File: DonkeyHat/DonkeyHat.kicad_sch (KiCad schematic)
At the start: 12 parts, among them J1 GPIO, J2 Encoder 2, J3 Encoder 1, U2 rp2040-zero

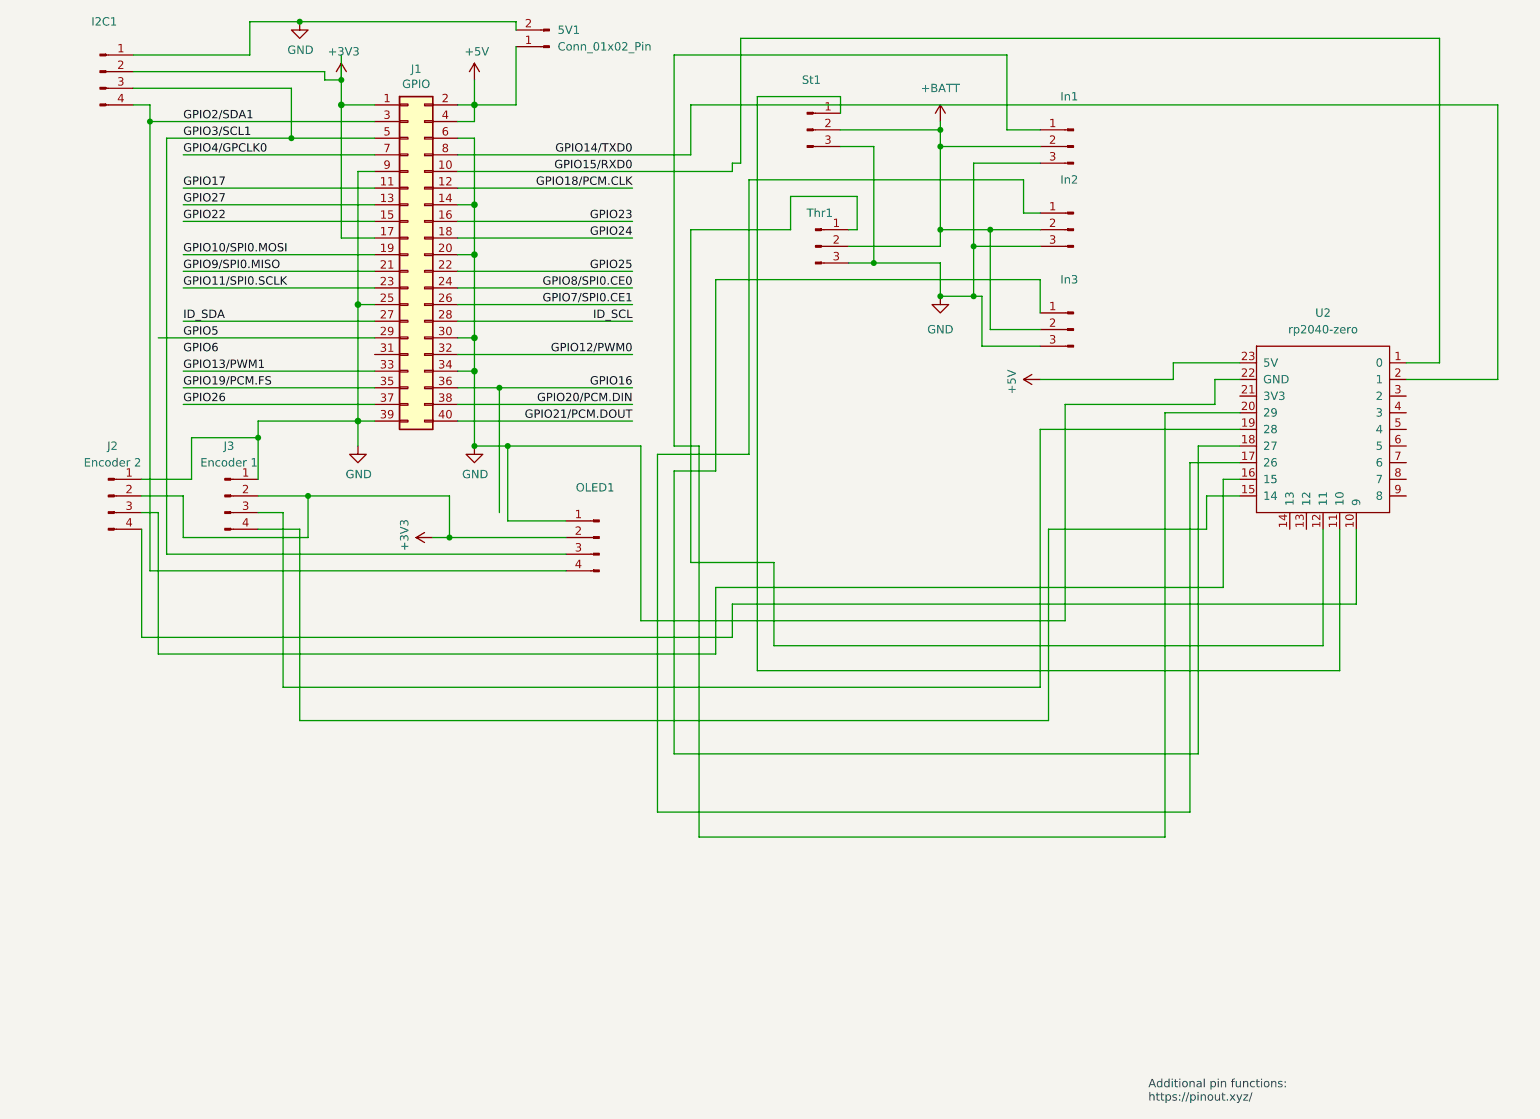
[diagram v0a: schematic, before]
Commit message: Typo
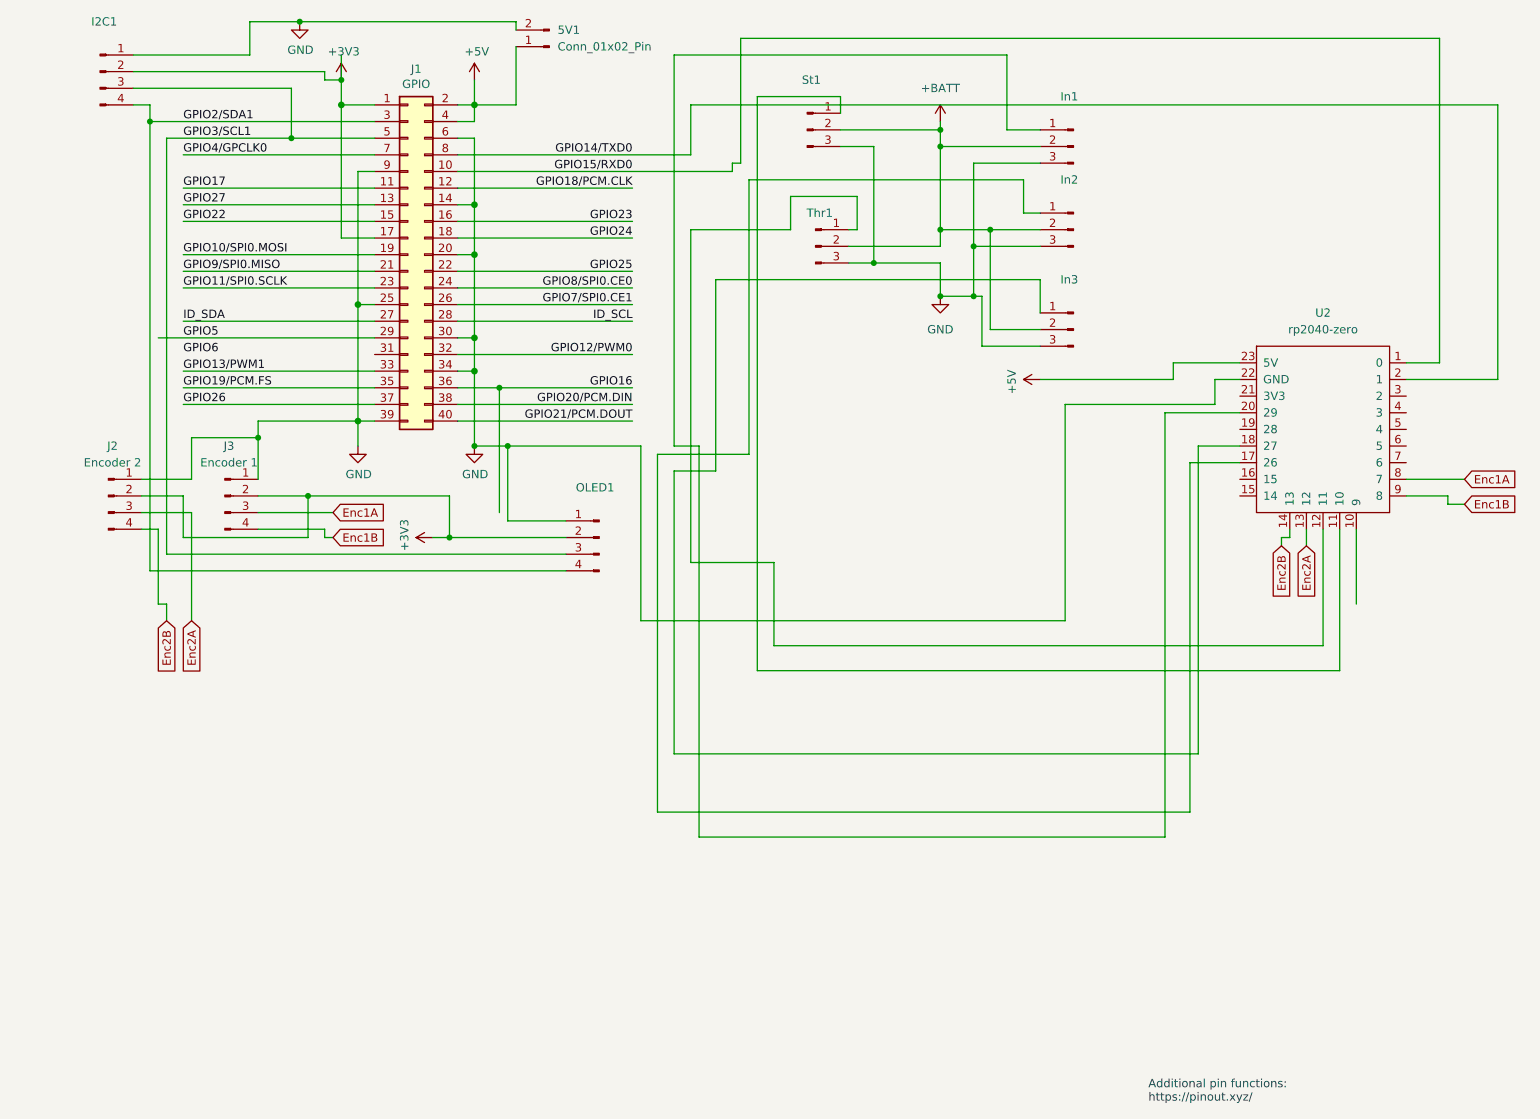
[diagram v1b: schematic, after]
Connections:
- net at U2.16 (15): no longer J2.3 (Pin_3)
- net at U2.10 (9): no longer J2.4 (Pin_4)
- net at U2.19 (28): no longer J3.3 (Pin_3)
- net at U2.15 (14): no longer J3.4 (Pin_4)
- net Enc2A: now reaches U2.13 (12)
- net Enc2A: now also J2.3 (Pin_3)
- net Enc2B: now reaches U2.14 (13)
- net Enc2B: now also J2.4 (Pin_4)
- net Enc1A: now reaches U2.8 (7)
- net Enc1A: now also J3.3 (Pin_3)
- net Enc1B: now reaches U2.9 (8)
- net Enc1B: now also J3.4 (Pin_4)

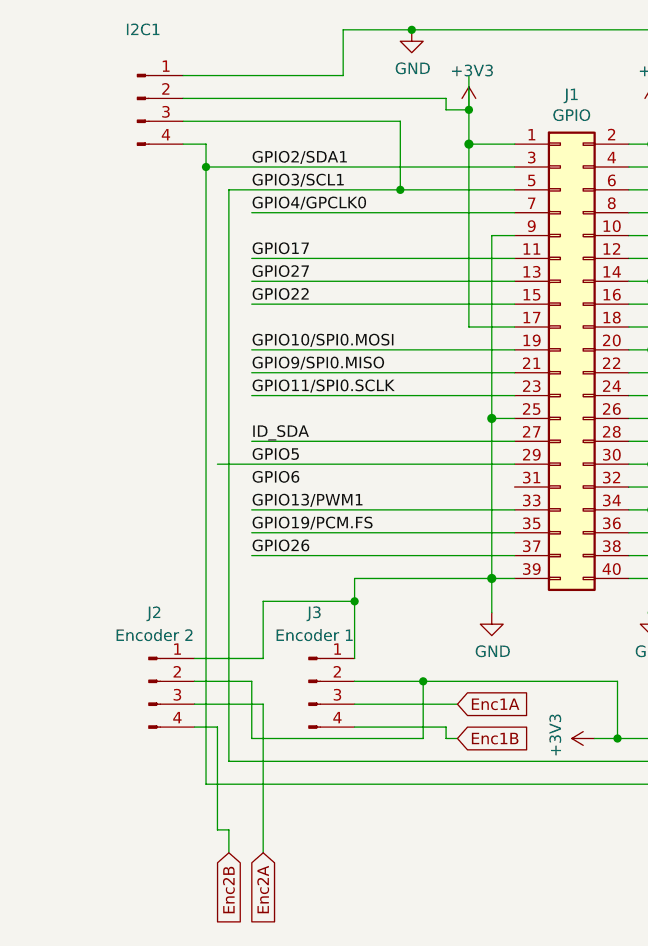
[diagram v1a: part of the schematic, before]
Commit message: New PCB
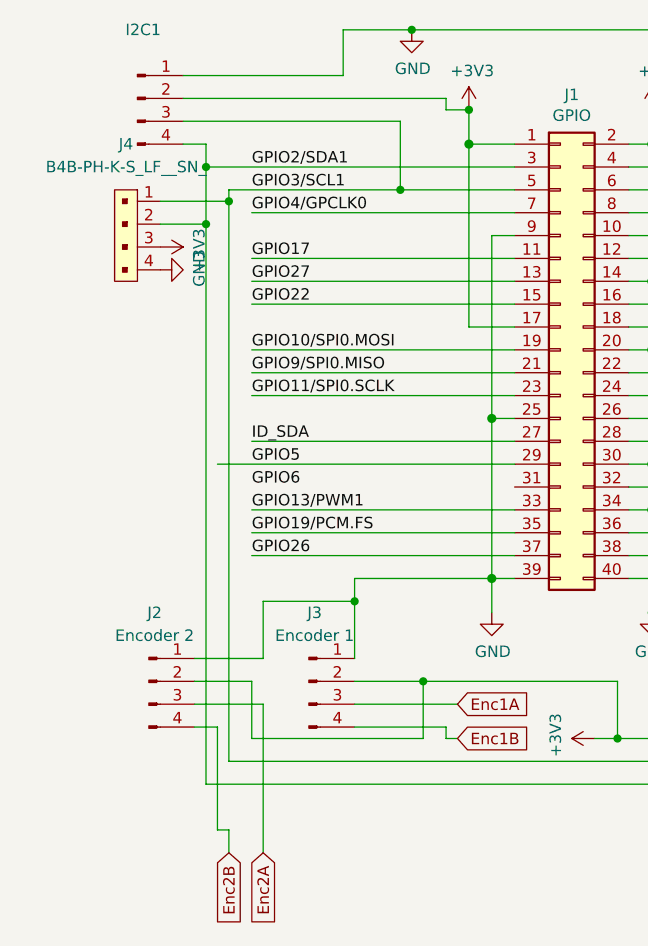
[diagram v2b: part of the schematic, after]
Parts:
- added J4: B4B-PH-K-S_LF__SN_, Connector_JST:JST_SH_BM04B-SRSS-TB_1x04-1MP_P1.00mm_Vertical, symbol dk_Rectangular-Connectors-Headers-Male-Pins:B4B-PH-K-S_LF__SN_
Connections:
- net +3V3: now also J4.3
- net GND: now also J4.4
- net GPIO2/SDA1: now also J4.2
- net GPIO3/SCL1: now also J4.1

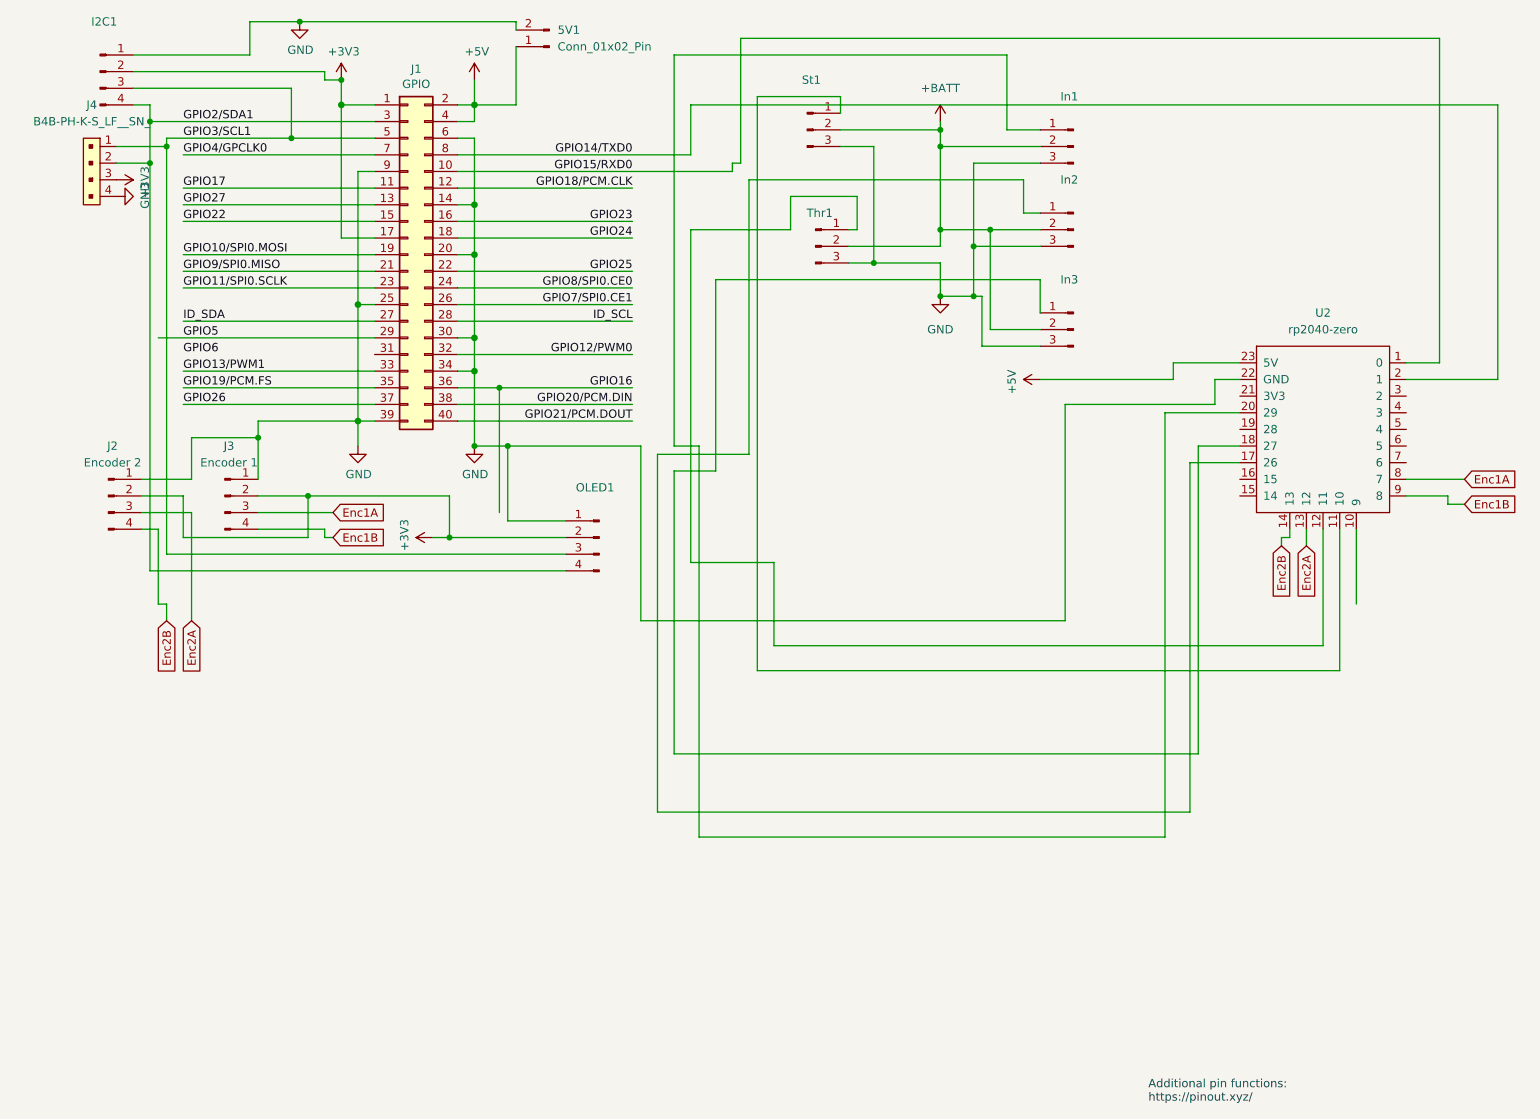
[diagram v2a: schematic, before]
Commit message: WIP
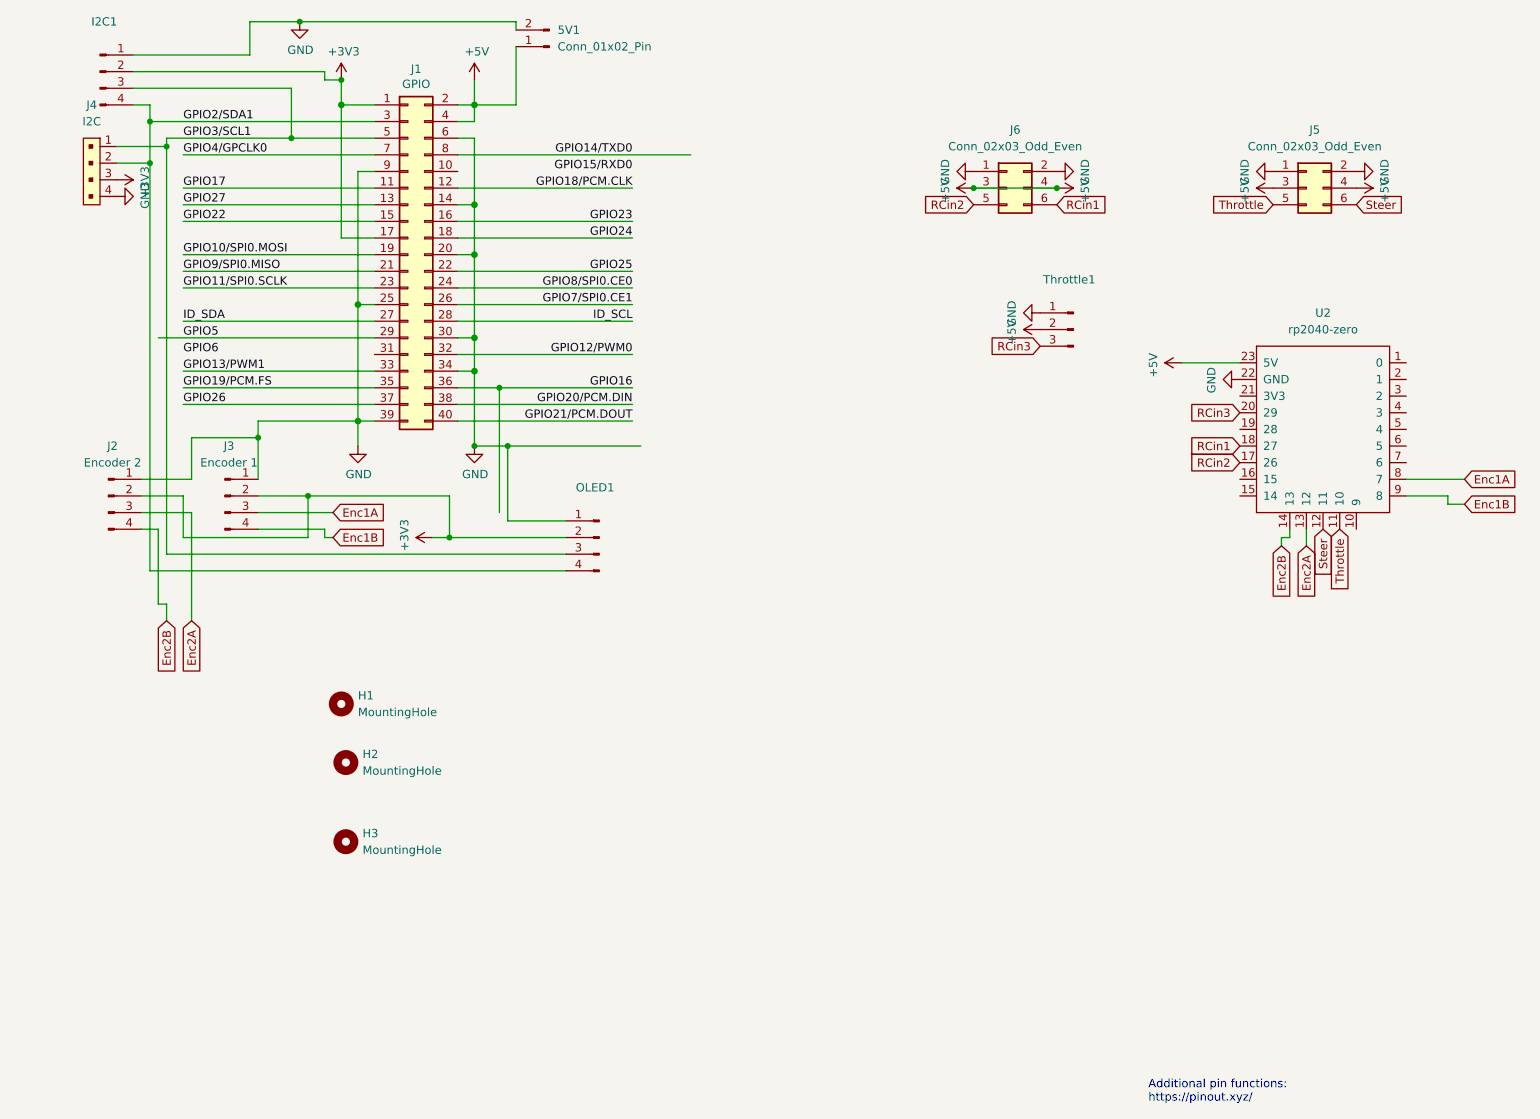
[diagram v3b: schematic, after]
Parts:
- removed In1: RC 1, Connector_PinHeader_2.54mm:PinHeader_1x03_P2.54mm_Vertical, symbol Connector:Conn_01x03_Pin
- removed In2, St1, Thr1: Conn_01x03_Pin, Connector_PinHeader_2.54mm:PinHeader_1x03_P2.54mm_Vertical, symbol Connector:Conn_01x03_Pin
- added H1, H2, H3: MountingHole, symbol Mechanical:MountingHole
- added J5, J6: Conn_02x03_Odd_Even, Connector_PinHeader_2.54mm:PinHeader_2x03_P2.54mm_Vertical, symbol Connector_Generic:Conn_02x03_Odd_Even
- J4: value B4B-PH-K-S_LF__SN_ -> I2C
- renumbered In3 to Throttle1
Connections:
- net +BATT is gone; now on net +5V: Throttle1.2 (Pin_2)
- net +5V: now also J5.3 (Pin_3), J5.4 (Pin_4), J6.3 (Pin_3), J6.4 (Pin_4)
- net GND: now also Throttle1.1 (Pin_1), J5.1 (Pin_1), J5.2 (Pin_2), J6.1 (Pin_1), J6.2 (Pin_2); no longer Throttle1.3 (Pin_3)
- net GPIO14/TXD0: no longer U2.2 (1)
- net GPIO15/RXD0: no longer J1.10 (Pin_10), U2.1 (0)
- net Steer: now reaches U2.12 (11)
- net Steer: now also J5.6 (Pin_6)
- net Throttle: now reaches U2.11 (10)
- net Throttle: now also J5.5 (Pin_5)
- net RCin2: now reaches U2.17 (26)
- net RCin2: now also J6.5 (Pin_5)
- net RCin1: now reaches U2.18 (27)
- net RCin1: now also J6.6 (Pin_6); no longer Throttle1.1 (Pin_1)
- net RCin3: now reaches U2.20 (29)
- net RCin3: now also Throttle1.3 (Pin_3)
